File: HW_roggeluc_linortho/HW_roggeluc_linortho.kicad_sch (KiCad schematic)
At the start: 13 parts, among them P1 ${SIM.PARAMS}, P2 ${SIM.PARAMS}

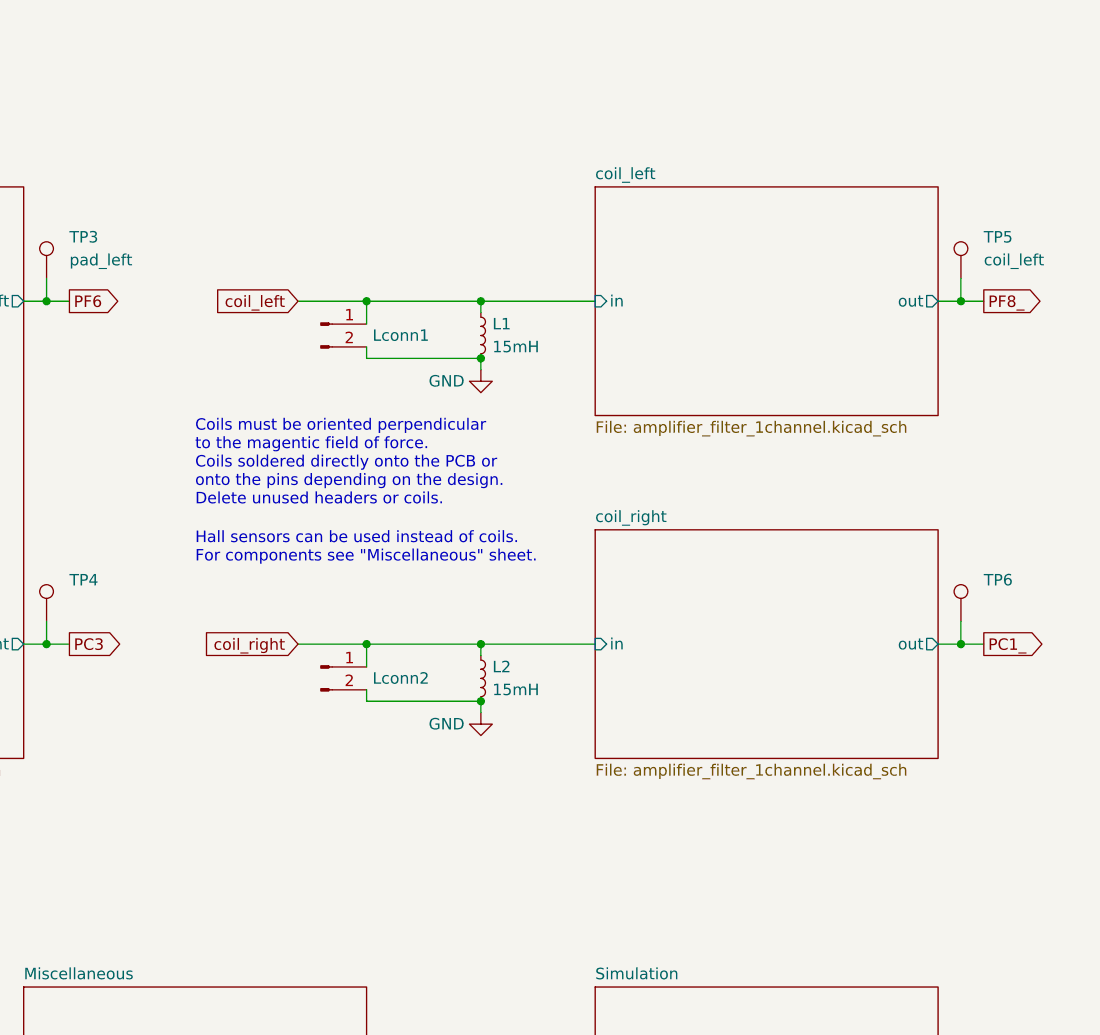
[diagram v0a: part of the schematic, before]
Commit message: OPAMP ANTENNA
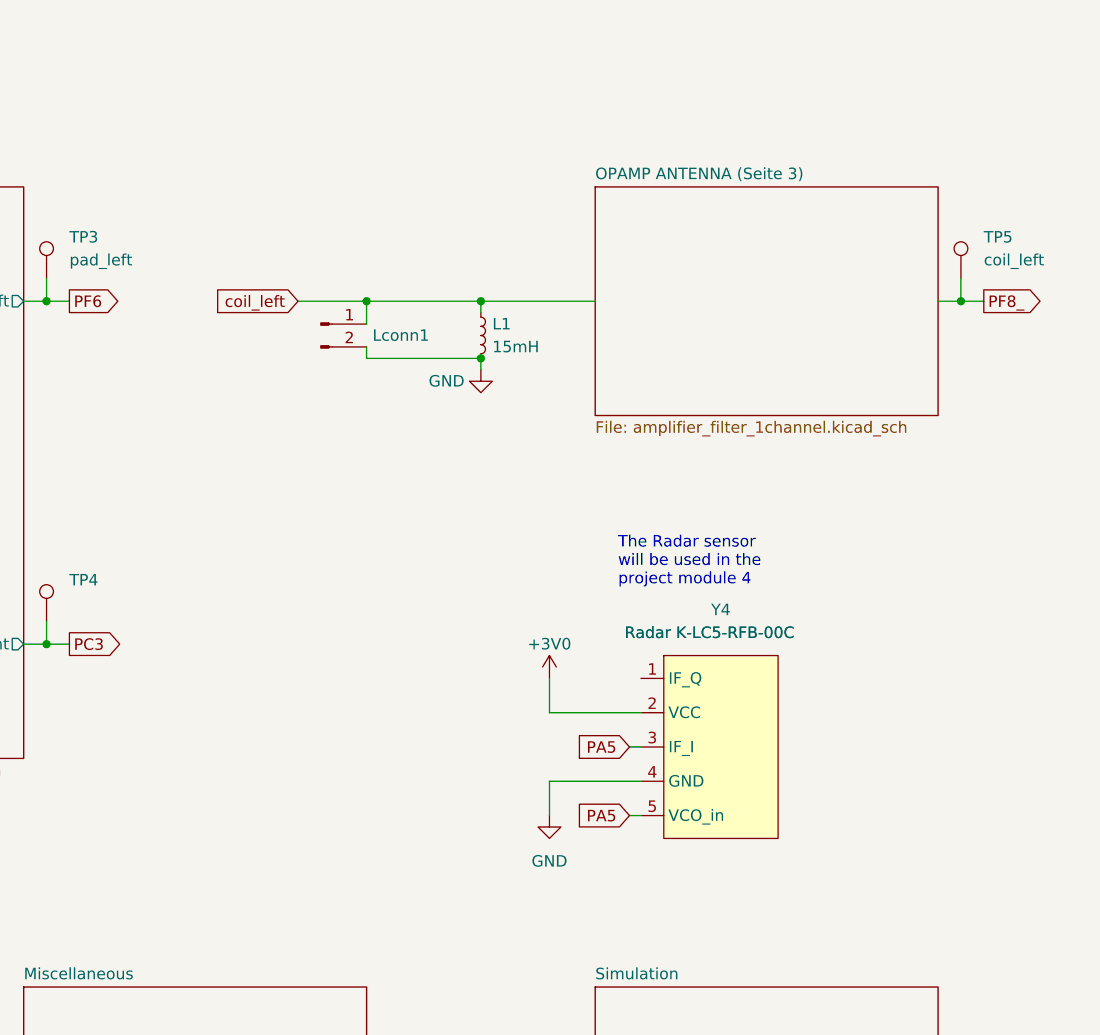
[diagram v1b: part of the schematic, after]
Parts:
- removed L2: 15mH, Inductor_SMD:L_Bourns_SRN6045TA, symbol Device:L_Small
- removed Lconn2: Conn_01x02_Male, Connector_PinHeader_2.54mm:PinHeader_1x02_P2.54mm_Vertical, symbol Connector:Conn_01x02_Pin
- removed TP6: ${SIM.PARAMS}, TestPoint:TestPoint_Loop_D2.60mm_Drill1.6mm_Beaded, symbol Connector:TestPoint
- added Y4: ${SIM.PARAMS}, HW_template:Radar_K-LC5, symbol HW_template:Radar K-LC5-RFB-00C
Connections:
- net +3V0: now also Y4.2 (VCC)
- net GND: now also Y4.4 (GND)
- net PA5: now also Y4.3 (IF_I), Y4.5 (VCO_in)
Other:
- sheet coil_left renamed OPAMP ANTENNA (Seite 3)
- removed sheet coil_right
- sheet OPAMP ANTENNA (Seite 3) ports: added none; removed in, out
- note added: "The Radar sensor will be used in the project module 4"
- note removed: "Coils must be oriented perpendicular to the magentic field of force. Coils soldered directly onto the PCB or onto the pins depending on the design. Delete unused headers or coils."
- note removed: "Hall sensors can be used instead of coils. For components see "Miscellaneous" sheet."

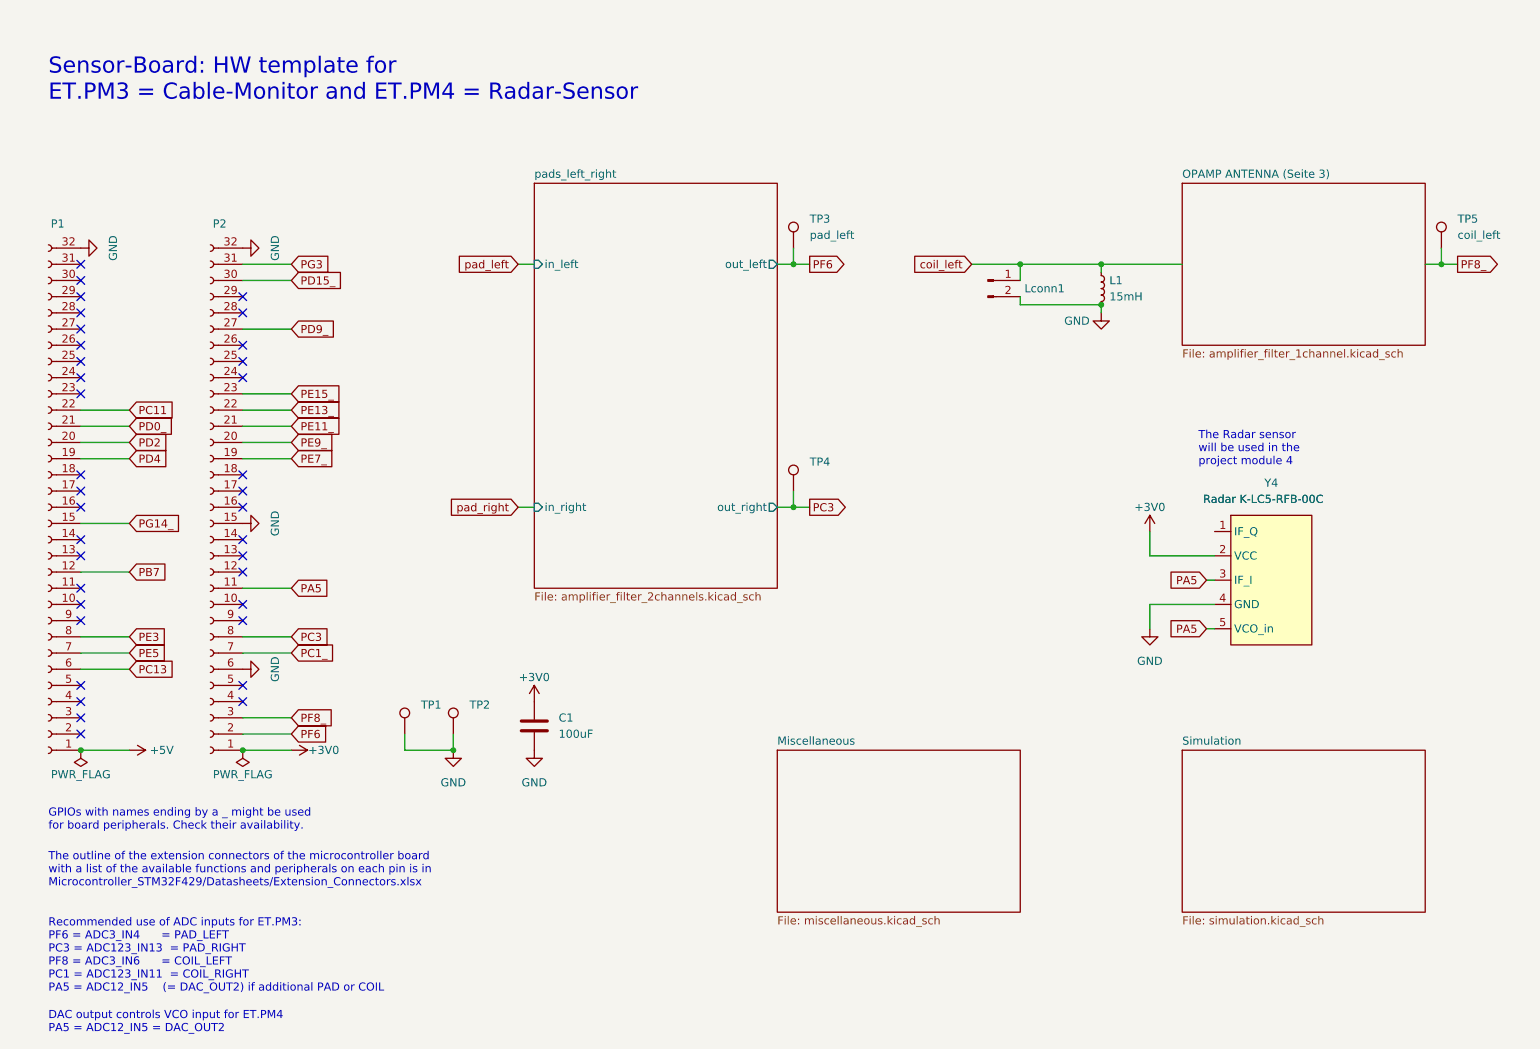
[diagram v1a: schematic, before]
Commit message: kek
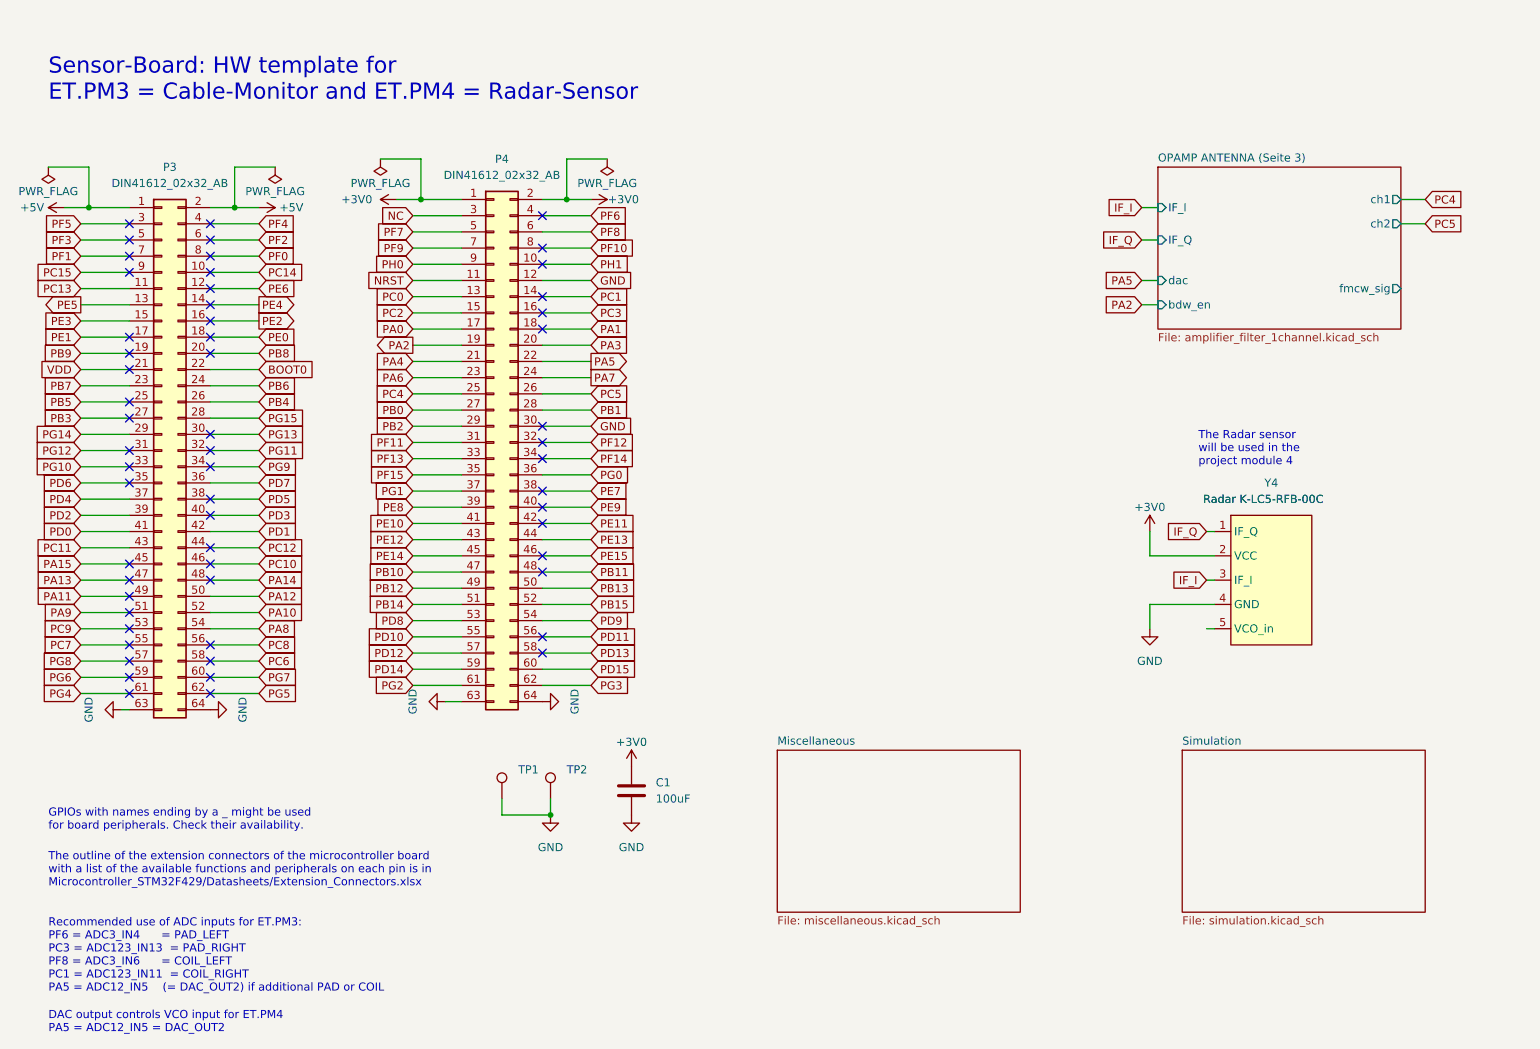
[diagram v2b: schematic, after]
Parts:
- removed L1: 15mH, Inductor_SMD:L_Bourns_SRN6045TA, symbol Device:L_Small
- removed Lconn1: Conn_01x02_Male, Connector_PinHeader_2.54mm:PinHeader_1x02_P2.54mm_Vertical, symbol Connector:Conn_01x02_Pin
- removed P1, P2: ${SIM.PARAMS}, Connector_PinSocket_2.54mm:PinSocket_1x32_P2.54mm_Vertical, symbol Connector:Conn_01x32_Socket
- removed TP3: pad_left, TestPoint:TestPoint_Loop_D2.60mm_Drill1.6mm_Beaded, symbol Connector:TestPoint
- removed TP4: ${SIM.PARAMS}, TestPoint:TestPoint_Loop_D2.60mm_Drill1.6mm_Beaded, symbol Connector:TestPoint
- removed TP5: coil_left, TestPoint:TestPoint_Loop_D2.60mm_Drill1.6mm_Beaded, symbol Connector:TestPoint
- added P3, P4: DIN41612_02x32_AB, Connector_PinSocket_2.54mm:PinSocket_2x32_P2.54mm_Vertical, symbol Connector:DIN41612_02x32_AB
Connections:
- net +3V0: now also P4.1 (Pin_a1), P4.2 (Pin_b1)
- net +5V: now also P3.1 (Pin_a1), P3.2 (Pin_b1)
- net GND: now also P3.63 (Pin_a32), P3.64 (Pin_b32), P4.12 (Pin_b6), P4.30 (Pin_b15), P4.63 (Pin_a32), P4.64 (Pin_b32)
- net PA5: now also P4.22 (Pin_b11); no longer Y4.3 (IF_I), Y4.5 (VCO_in)
- net PB7: now also P3.23 (Pin_a12)
- net PC11: now also P3.43 (Pin_a22)
- net PC13: now also P3.11 (Pin_a6)
- net PC3: now also P4.16 (Pin_b8)
- net PD2: now also P3.39 (Pin_a20)
- net PD4: now also P3.37 (Pin_a19)
- net PE3: now also P3.15 (Pin_a8)
- net PE5: now also P3.13 (Pin_a7)
- net PF6: now also P4.4 (Pin_b2)
- net PG3: now also P4.62 (Pin_b31)
- net IF_Q: now reaches Y4.1 (IF_Q)
- new net BOOT0: P3.22 (Pin_b11)
- new net IF_I: Y4.3 (IF_I)
- new net NC: P4.3 (Pin_a2)
- new net NRST: P4.11 (Pin_a6)
- new net PA0: P4.17 (Pin_a9)
- new net PA1: P4.18 (Pin_b9)
- new net PA10: P3.52 (Pin_b26)
- new net PA11: P3.49 (Pin_a25)
- new net PA12: P3.50 (Pin_b25)
- new net PA13: P3.47 (Pin_a24)
- new net PA14: P3.48 (Pin_b24)
- new net PA15: P3.45 (Pin_a23)
- new net PA2: P4.19 (Pin_a10)
- new net PA3: P4.20 (Pin_b10)
- new net PA4: P4.21 (Pin_a11)
- new net PA6: P4.23 (Pin_a12)
- new net PA7: P4.24 (Pin_b12)
- new net PA8: P3.54 (Pin_b27)
- new net PA9: P3.51 (Pin_a26)
- new net PB0: P4.27 (Pin_a14)
- new net PB1: P4.28 (Pin_b14)
- new net PB10: P4.47 (Pin_a24)
- new net PB11: P4.48 (Pin_b24)
- new net PB12: P4.49 (Pin_a25)
- new net PB13: P4.50 (Pin_b25)
- new net PB14: P4.51 (Pin_a26)
- new net PB15: P4.52 (Pin_b26)
- new net PB2: P4.29 (Pin_a15)
- new net PB3: P3.27 (Pin_a14)
- new net PB4: P3.26 (Pin_b13)
- new net PB5: P3.25 (Pin_a13)
- new net PB6: P3.24 (Pin_b12)
- new net PB8: P3.20 (Pin_b10)
- new net PB9: P3.19 (Pin_a10)
- new net PC0: P4.13 (Pin_a7)
- new net PC1: P4.14 (Pin_b7)
- new net PC10: P3.46 (Pin_b23)
- new net PC12: P3.44 (Pin_b22)
- new net PC14: P3.10 (Pin_b5)
- new net PC15: P3.9 (Pin_a5)
- new net PC2: P4.15 (Pin_a8)
- new net PC4: P4.25 (Pin_a13)
- new net PC5: P4.26 (Pin_b13)
- new net PC6: P3.58 (Pin_b29)
- new net PC7: P3.55 (Pin_a28)
- new net PC8: P3.56 (Pin_b28)
- new net PC9: P3.53 (Pin_a27)
- new net PD0: P3.41 (Pin_a21)
- new net PD1: P3.42 (Pin_b21)
- new net PD10: P4.55 (Pin_a28)
- new net PD11: P4.56 (Pin_b28)
- new net PD12: P4.57 (Pin_a29)
- new net PD13: P4.58 (Pin_b29)
- new net PD14: P4.59 (Pin_a30)
- new net PD15: P4.60 (Pin_b30)
- new net PD3: P3.40 (Pin_b20)
- new net PD5: P3.38 (Pin_b19)
- new net PD6: P3.35 (Pin_a18)
- new net PD7: P3.36 (Pin_b18)
- new net PD8: P4.53 (Pin_a27)
- new net PD9: P4.54 (Pin_b27)
- new net PE0: P3.18 (Pin_b9)
- new net PE1: P3.17 (Pin_a9)
- new net PE10: P4.41 (Pin_a21)
- new net PE11: P4.42 (Pin_b21)
- new net PE12: P4.43 (Pin_a22)
- new net PE13: P4.44 (Pin_b22)
- new net PE14: P4.45 (Pin_a23)
- new net PE15: P4.46 (Pin_b23)
- new net PE2: P3.16 (Pin_b8)
- new net PE4: P3.14 (Pin_b7)
- new net PE6: P3.12 (Pin_b6)
- new net PE7: P4.38 (Pin_b19)
- new net PE8: P4.39 (Pin_a20)
- new net PE9: P4.40 (Pin_b20)
- new net PF0: P3.8 (Pin_b4)
- new net PF1: P3.7 (Pin_a4)
- new net PF10: P4.8 (Pin_b4)
- new net PF11: P4.31 (Pin_a16)
- new net PF12: P4.32 (Pin_b16)
- new net PF13: P4.33 (Pin_a17)
- new net PF14: P4.34 (Pin_b17)
- new net PF15: P4.35 (Pin_a18)
- new net PF2: P3.6 (Pin_b3)
- new net PF3: P3.5 (Pin_a3)
- new net PF4: P3.4 (Pin_b2)
- new net PF5: P3.3 (Pin_a2)
- new net PF7: P4.5 (Pin_a3)
- new net PF8: P4.6 (Pin_b3)
- new net PF9: P4.7 (Pin_a4)
- new net PG0: P4.36 (Pin_b18)
- new net PG1: P4.37 (Pin_a19)
- new net PG10: P3.33 (Pin_a17)
- new net PG11: P3.32 (Pin_b16)
- new net PG12: P3.31 (Pin_a16)
- new net PG13: P3.30 (Pin_b15)
- new net PG14: P3.29 (Pin_a15)
- new net PG15: P3.28 (Pin_b14)
- new net PG2: P4.61 (Pin_a31)
- new net PG4: P3.61 (Pin_a31)
- new net PG5: P3.62 (Pin_b31)
- new net PG6: P3.59 (Pin_a30)
- new net PG7: P3.60 (Pin_b30)
- new net PG8: P3.57 (Pin_a29)
- new net PG9: P3.34 (Pin_b17)
- new net PH0: P4.9 (Pin_a5)
- new net PH1: P4.10 (Pin_b5)
- new net VDD: P3.21 (Pin_a11)
- no-connect marks 36 -> 58
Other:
- removed sheet pads_left_right
- sheet OPAMP ANTENNA (Seite 3) ports: added IF_I, IF_Q, bdw_en, ch1, ch2, dac, fmcw_sig; removed none
- moved on the sheet: C1, TP1, TP2

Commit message: lol
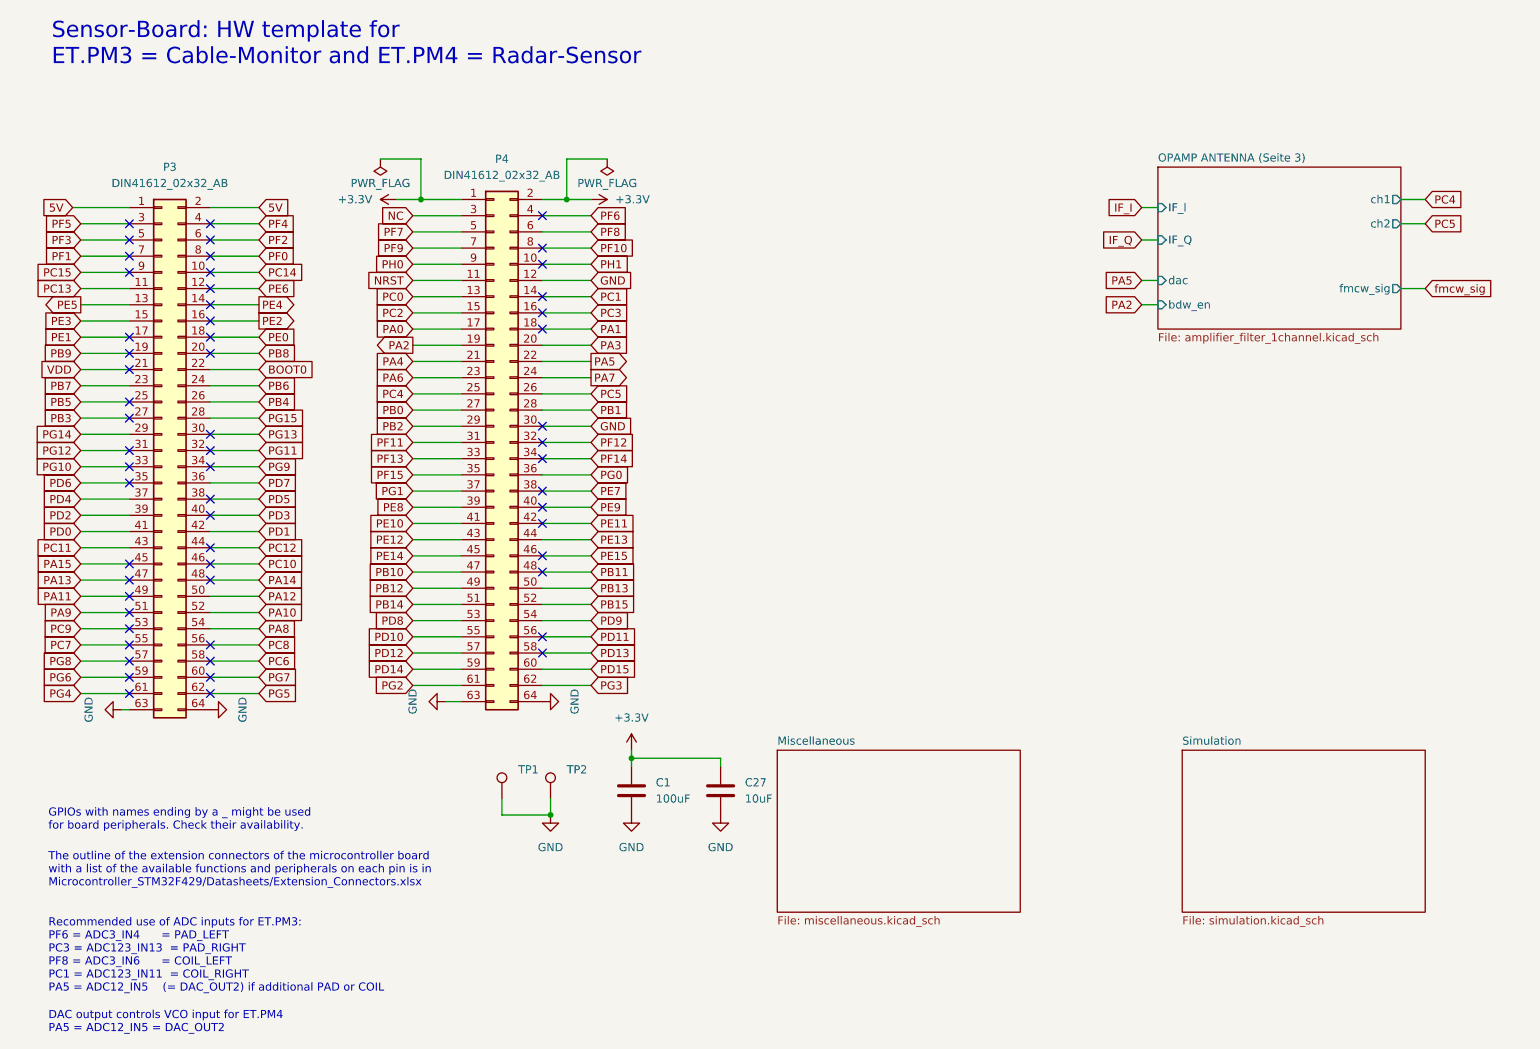
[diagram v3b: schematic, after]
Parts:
- removed Y4: ${SIM.PARAMS}, HW_template:Radar_K-LC5, symbol HW_template:Radar K-LC5-RFB-00C
- added C27: 10uF, Capacitor_SMD:C_0805_2012Metric_Pad1.18x1.45mm_HandSolder, symbol Device:C
- C1: footprint Capacitor_SMD:C_1206_3216Metric_Pad1.33x1.80mm_HandSolder -> Capacitor_SMD:C_0805_2012Metric_Pad1.18x1.45mm_HandSolder
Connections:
- net GND: now also C27.2
- net +3V0 renamed +3.3V
- net +3.3V: now also C27.1
- net +5V renamed 5V
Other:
- note removed: "The Radar sensor will be used in the project module 4"
